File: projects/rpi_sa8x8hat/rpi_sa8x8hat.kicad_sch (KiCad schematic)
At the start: 37 parts, among them J1 RPi_GPIO, U1 SA818, U2 TLV320AIC3204, U3 AT24CS32-STUM

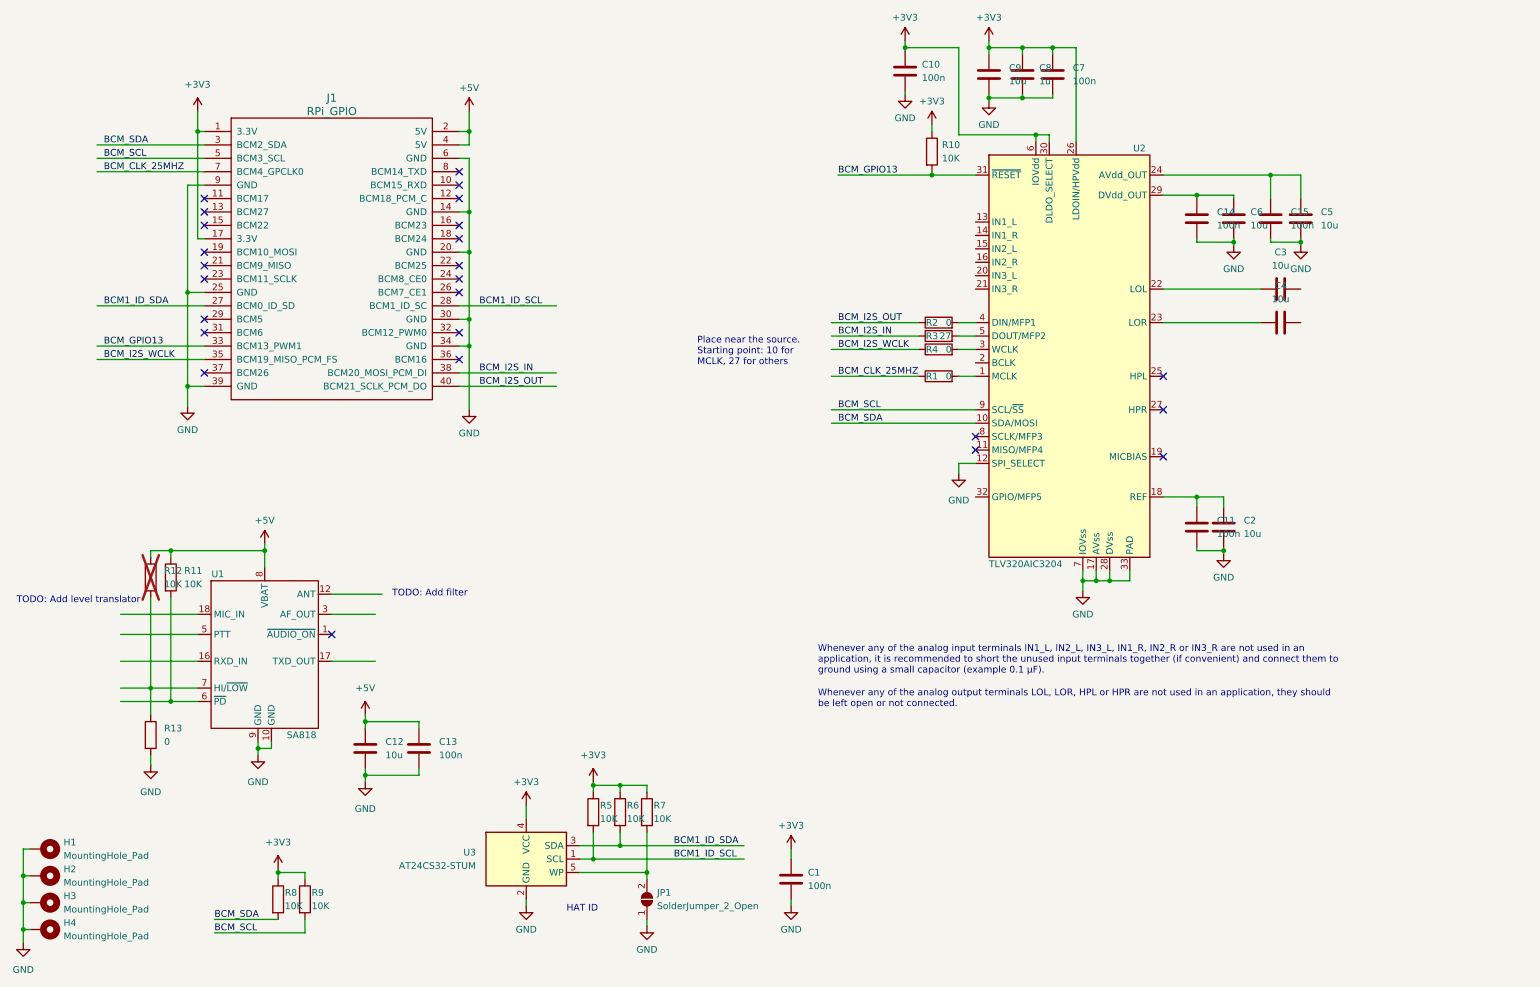
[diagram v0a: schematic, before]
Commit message: wip
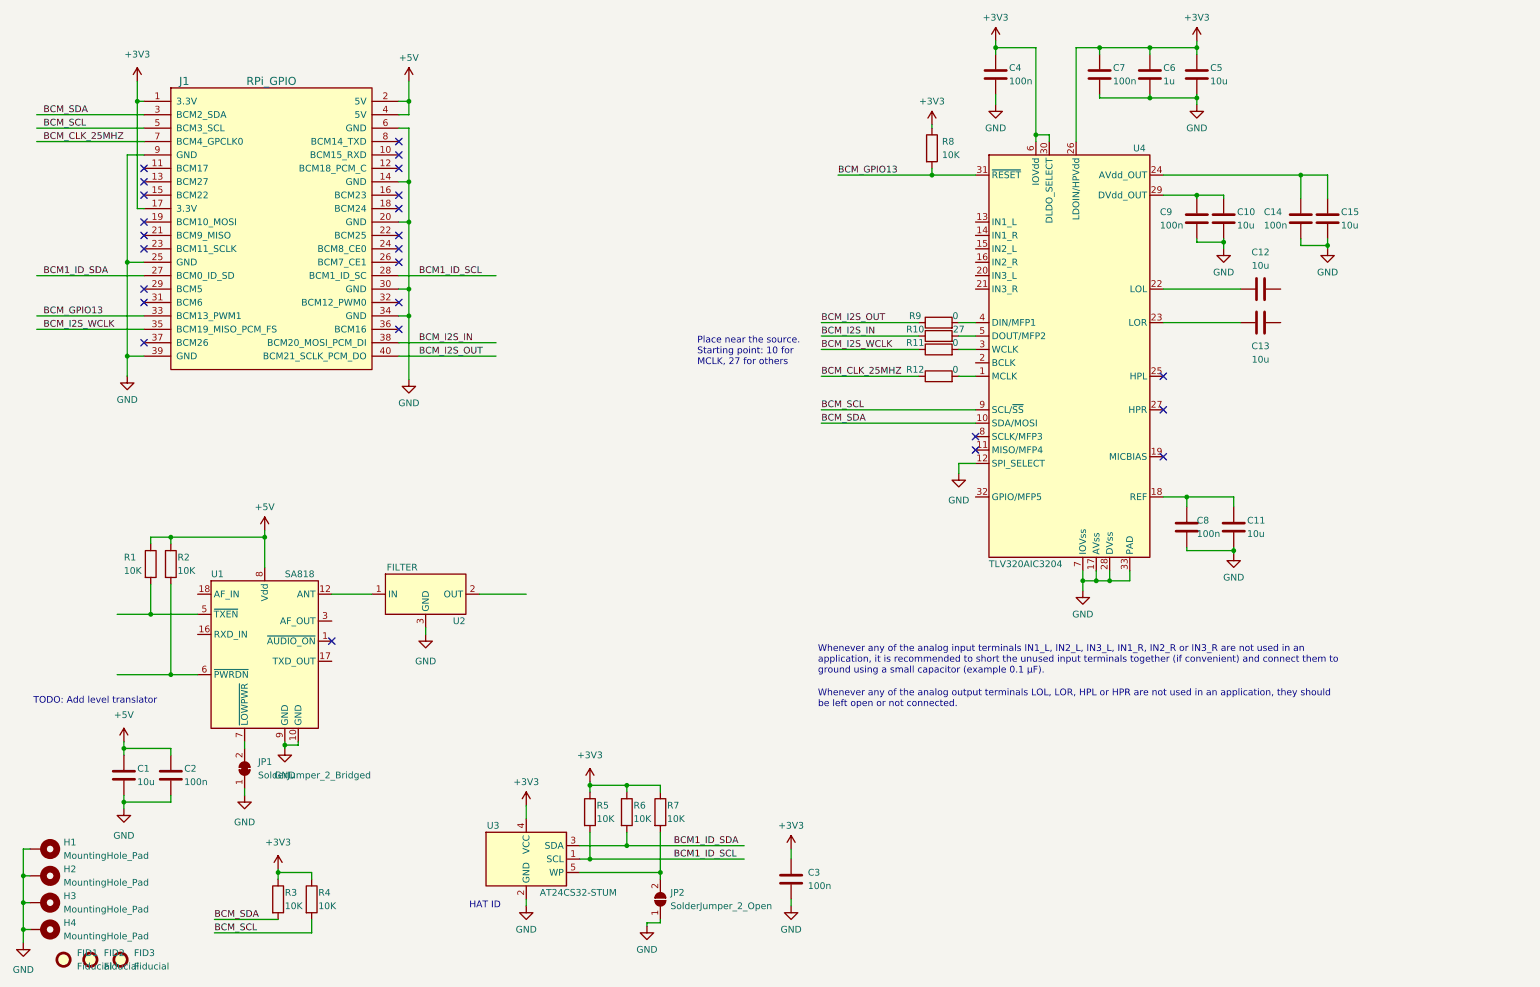
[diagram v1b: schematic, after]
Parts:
- removed R12: 10K, symbol Device:R
- removed R13: 0, symbol Device:R
- added FID1, FID2, FID3: Fiducial, symbol Mechanical:Fiducial
- added JP1: SolderJumper_2_Bridged, symbol Jumper:SolderJumper_2_Bridged
- added R1: 10K, symbol Device:R
- added U2: FILTER, symbol rpi_s8x8hat:FILTER-3TERM
- J1: symbol rpi_sa8x8hat:RPi_GPIO -> rpi_s8x8hat:RPi_GPIO
- U1: footprint rpi_sa8x8hat:SA818 -> (none)
- renumbered C12 to C1, C6 to C10, C2 to C11, C3 to C12, C4 to C13, C15 to C14, C5 to C15, C13 to C2, C1 to C3, C10 to C4, C9 to C5, C8 to C6, C11 to C8, C14 to C9, JP1 to JP2, R3 to R10, R4 to R11, R1 to R12, R11 to R2, R8 to R3, R9 to R4, R10 to R8, R2 to R9, U2 to U4
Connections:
- net +5V: now also R1.1
- net GND: now also JP1.1 (A), U2.3 (GND)
- net at U1.7 (~{LOWPWR}): now also JP1.2 (B)
- net at U1.12 (ANT): now also U2.1 (IN)
- net at U1.5 (~{TXEN}): now also R1.2
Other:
- note removed: "TODO: Add filter"
- company: (none) -> Murgatroid Heavy Industries, LLC
- title: (none) -> RPi SA818 Hat
- moved on the sheet: C1, C10, C11, C12, C13, C14, C15, C2, C4, C5, C6, C7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

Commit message: wip
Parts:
- FID1, FID2, FID3: footprint (none) -> Fiducial:Fiducial_0.5mm_Mask1.5mm
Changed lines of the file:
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@@
       (effects (font (size 1.27 1.27)) (justify left))
     )
-    (property "Footprint" "" (at 34.925 192.405 0)
+    (property "Footprint" "Fiducial:Fiducial_0.5mm_Mask1.5mm" (at 34.925 192.405 0)
       (effects (font (size 1.27 1.27)) hide)
     )
@@
       (effects (font (size 1.27 1.27)) (justify left))
     )
-    (property "Footprint" "" (at 24.13 192.405 0)
+    (property "Footprint" "Fiducial:Fiducial_0.5mm_Mask1.5mm" (at 24.13 192.405 0)
       (effects (font (size 1.27 1.27)) hide)
     )
@@
       (effects (font (size 1.27 1.27)) (justify left))
     )
-    (property "Footprint" "" (at 29.21 192.405 0)
-      (effects (font (size 1.27 1.27)) hide)
-    )
+    (property "Footprint" "Fiducial:Fiducial_0.5mm_Mask1.5mm" (at 29.21 192.405 0)
+      (effects (font (size 1.27 1.27)) hide)
+    )
